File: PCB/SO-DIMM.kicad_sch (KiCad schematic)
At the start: 1 part, among them J1 SODIMM-260_Split

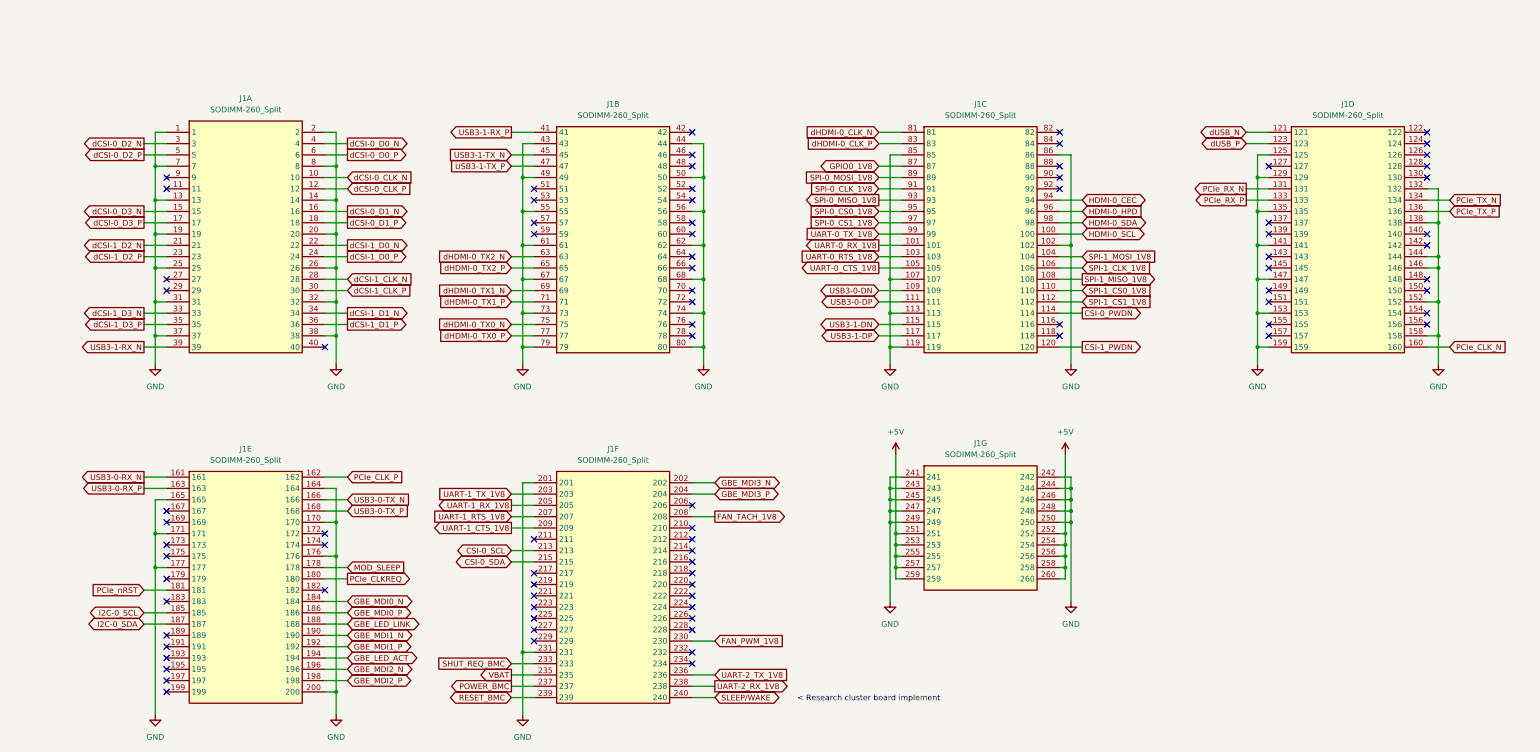
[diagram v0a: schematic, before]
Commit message: updated 2
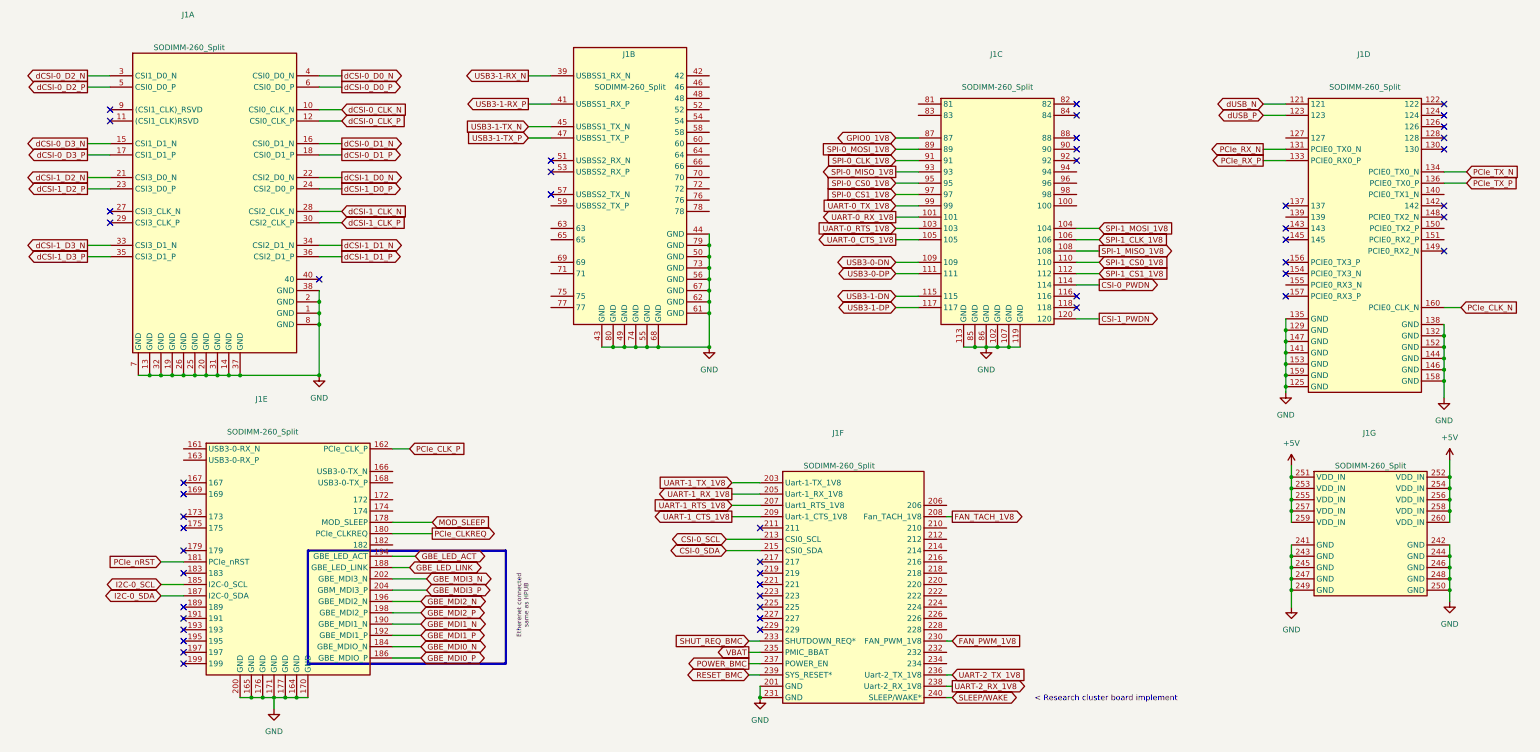
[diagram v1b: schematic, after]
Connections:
- net GBE_MDI3_N: now also J1.202 (GBE_MDI3_N); no longer J1.202
- net GBE_MDI3_P: now also J1.204 (GBM_MDI3_P); no longer J1.204
- net USB3-1-RX_N: now also J1.39 (USBSS1_RX_N); no longer J1.39
- net HDMI-0_CEC: no longer names the net of J1.94
- net HDMI-0_HPD: no longer names the net of J1.96
- net HDMI-0_SCL: no longer names the net of J1.100
- net HDMI-0_SDA: no longer names the net of J1.98
- net USB3-0-RX_N: no longer names the net of J1.161 (USB3-0-RX_N)
- net USB3-0-RX_P: no longer names the net of J1.163 (USB3-0-RX_P)
- net USB3-0-TX_N: no longer names the net of J1.166 (USB3-0-TX_N)
- net USB3-0-TX_P: no longer names the net of J1.168 (USB3-0-TX_P)
- net dHDMI-0_CLK_N: no longer names the net of J1.81
- net dHDMI-0_CLK_P: no longer names the net of J1.83
- net dHDMI-0_TX0_N: no longer names the net of J1.75
- net dHDMI-0_TX0_P: no longer names the net of J1.77
- net dHDMI-0_TX1_N: no longer names the net of J1.69
- net dHDMI-0_TX1_P: no longer names the net of J1.71
- net dHDMI-0_TX2_N: no longer names the net of J1.63
- net dHDMI-0_TX2_P: no longer names the net of J1.65
- no-connect marks 85 -> 49
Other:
- note added: "Etherenet connected same as HPUB"
